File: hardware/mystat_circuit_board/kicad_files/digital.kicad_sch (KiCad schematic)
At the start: 28 parts, among them J2 2173157-3, P1 ICSP, U5 PIC16F1459, U6 ADR421, U7 MCP3550-60, U8 MCP3550-60, U9 DAC1220, X1 2.5 MHz

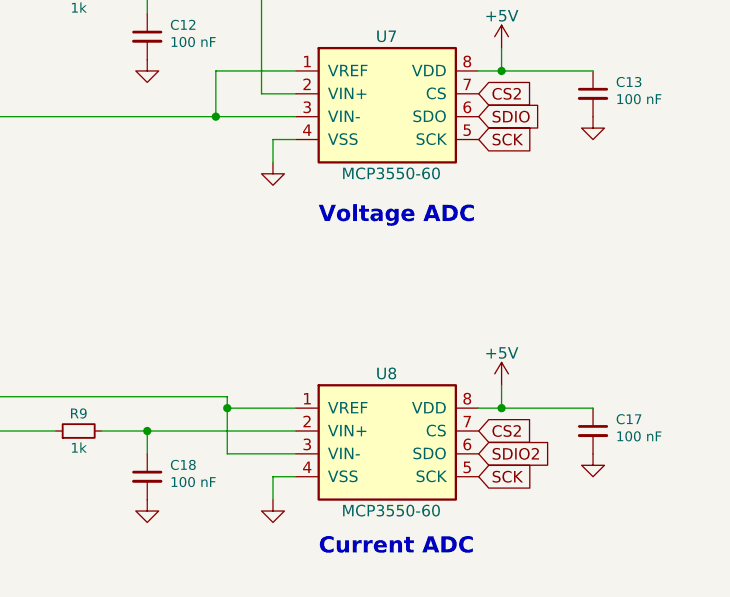
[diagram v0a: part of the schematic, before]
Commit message: merged Daniel's changes in to GUI. getting things ready in KiCAD 10 and finding substitute parts
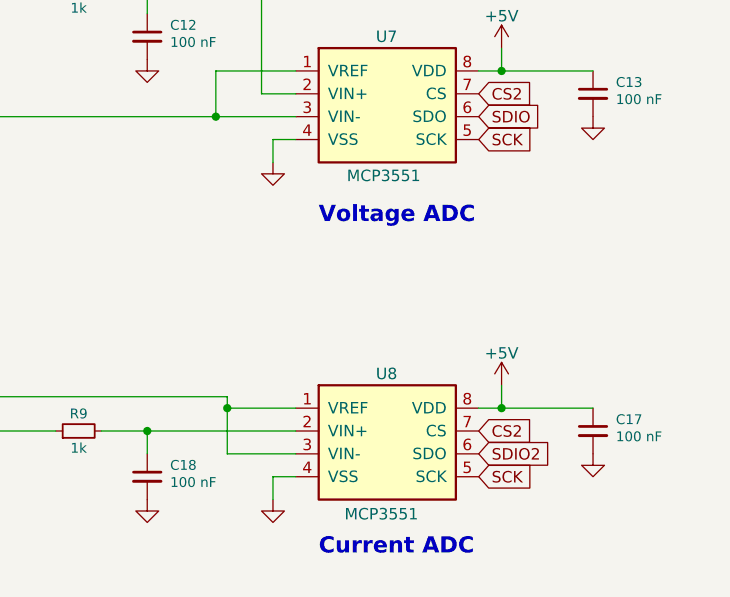
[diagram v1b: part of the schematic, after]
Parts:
- C16: LCSC (none) -> C138687; Part Number CL32B106KBJNNWE -> CL32B106KBJNNNE
- FB1: LCSC (none) -> C6968654; Part Number * -> ILBB0805ER320V
- J2: LCSC (none) -> C3197930
- P1: LCSC (none) -> C37208; Manufacturer Sullins Connector Solutions -> BOOMELE; Part Number PRPC006SAAN-RC -> 2.54-1x6PStraight pin
- R7, R9: LCSC (none) -> C17513; Manufacturer Yageo -> UNI-ROYAL; Part Number RC0805FR-071KL -> 0805W8F1001T5E
- R8: LCSC (none) -> C17414; Manufacturer Yageo -> UNI-ROYAL; Part Number RC0805FR-0710KL -> 0805W8F1002T5E
- U5: LCSC (none) -> C643250
- U6: LCSC (none) -> C9650; Part Number ADR421ARZ -> ADR421ARZ-REEL7
- U7, U8: value MCP3550-60 -> MCP3551; LCSC (none) -> C1520170; Part Number MCP3550-60E/SN -> MCP3551-E/SN
- U9: LCSC (none) -> C2679558; Part Number DAC1220E -> DAC1220E/2K5
- X1: LCSC (none) -> C2636517; Part Number ECS-25-S-1X -> ECS-25-S-1

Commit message: revert to KiCAD 10 state before attempting reed relay changes, to merge into master
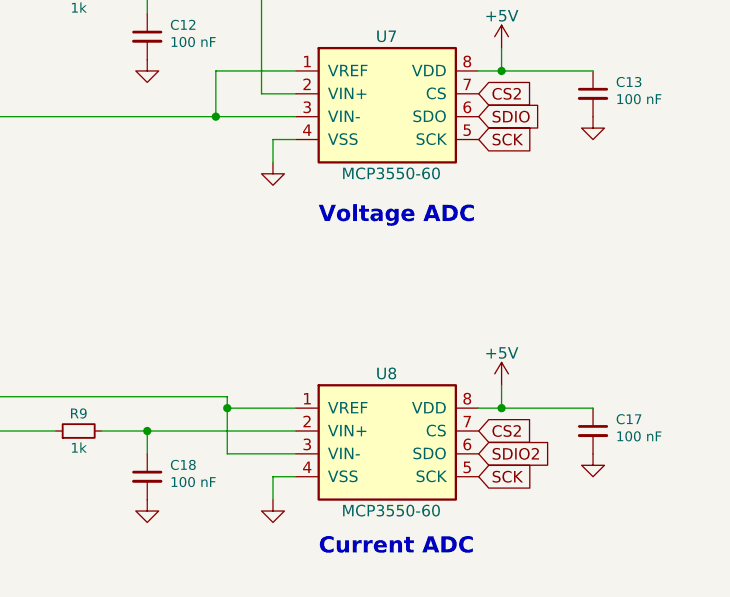
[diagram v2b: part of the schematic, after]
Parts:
- C16: LCSC C138687 -> (none); Part Number CL32B106KBJNNNE -> CL32B106KBJNNWE
- FB1: LCSC C6968654 -> (none); Part Number ILBB0805ER320V -> *
- J2: LCSC C3197930 -> (none)
- P1: LCSC C37208 -> (none); Manufacturer BOOMELE -> Sullins Connector Solutions; Part Number 2.54-1x6PStraight pin -> PRPC006SAAN-RC
- R7, R9: LCSC C17513 -> (none); Manufacturer UNI-ROYAL -> Yageo; Part Number 0805W8F1001T5E -> RC0805FR-071KL
- R8: LCSC C17414 -> (none); Manufacturer UNI-ROYAL -> Yageo; Part Number 0805W8F1002T5E -> RC0805FR-0710KL
- U5: LCSC C643250 -> (none)
- U6: LCSC C9650 -> (none); Part Number ADR421ARZ-REEL7 -> ADR421ARZ
- U7, U8: value MCP3551 -> MCP3550-60; LCSC C1520170 -> (none); Part Number MCP3551-E/SN -> MCP3550-60E/SN
- U9: LCSC C2679558 -> (none); Part Number DAC1220E/2K5 -> DAC1220E
- X1: LCSC C2636517 -> (none); Part Number ECS-25-S-1 -> ECS-25-S-1X
